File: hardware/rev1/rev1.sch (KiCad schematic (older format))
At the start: 28 parts, among them U1 BNO055, U2 MPL3115A2, U3 Teensy3.6, Y1 Crystal_32kHz768

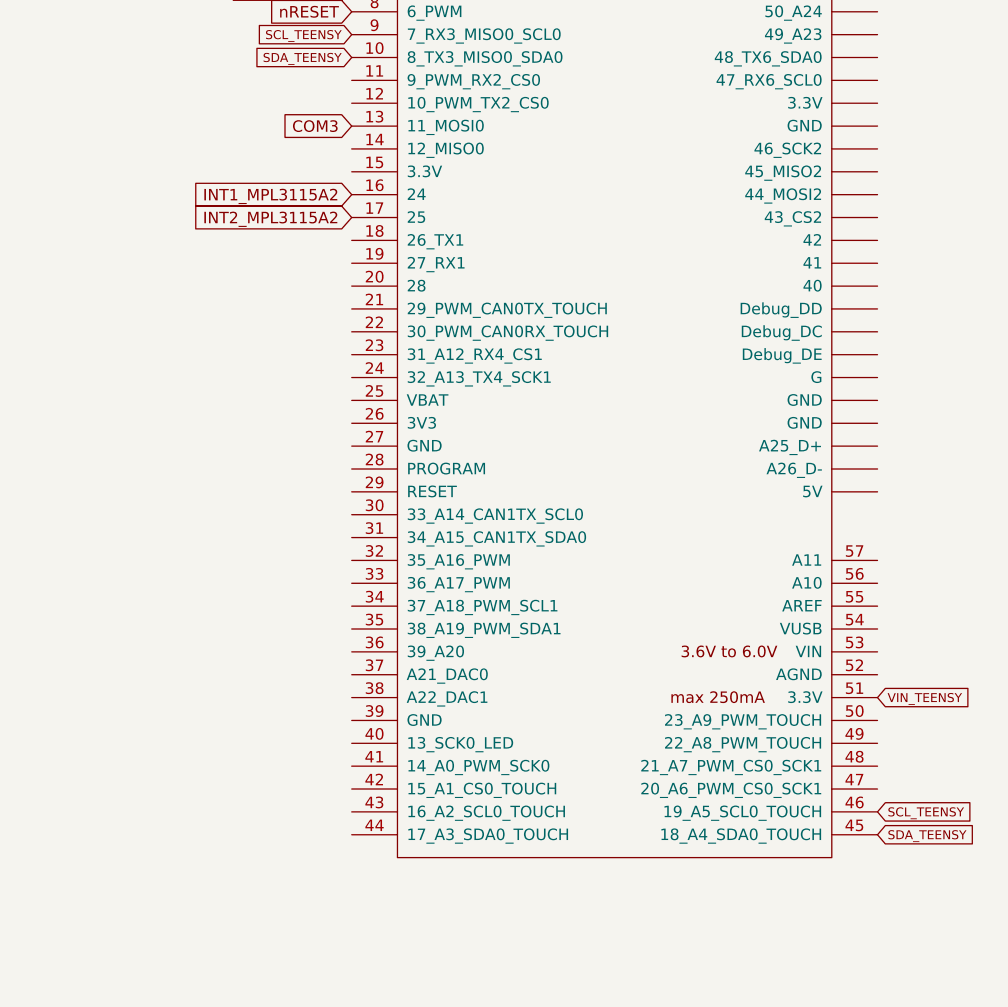
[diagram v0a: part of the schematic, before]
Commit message: wip
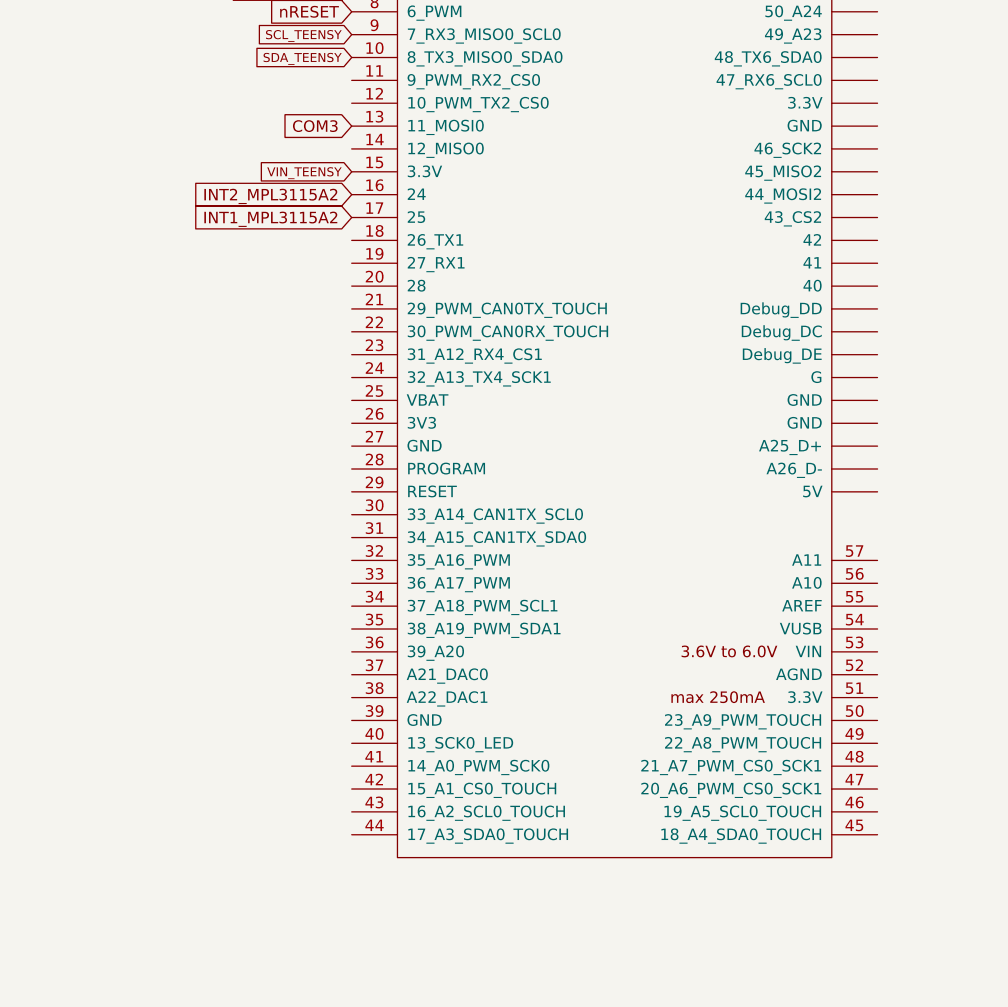
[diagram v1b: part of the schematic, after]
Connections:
- net +3V3: now also U3.15 (3.3V); no longer U3.51 (3.3V)
- net INT1_MPL3115A2: now also U3.17 (25); no longer U3.16 (24)
- net INT2_MPL3115A2: now also U3.16 (24); no longer U3.17 (25)
- net SCL_TEENSY: no longer U3.46 (19_A5_SCL0_TOUCH)
- net SDA_TEENSY: no longer U3.45 (18_A4_SDA0_TOUCH)
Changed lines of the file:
@@
 Text Label 27400 2800 2    118  ~ 0
 GND
-Text GLabel 29700 6500 2    39   Input ~ 0
+Text GLabel 27400 4200 0    39   Input ~ 0
 VIN_TEENSY
-Text GLabel 29700 7100 2    39   Input ~ 0
-SDA_TEENSY
-Text GLabel 29700 7000 2    39   Input ~ 0
-SCL_TEENSY
 Wire Wire Line
 	6900 7300 9850 7300
 Text GLabel 9850 7300 2    50   Input ~ 0
 INT_BNO055
+Text GLabel 27400 4400 0    50   Input ~ 0
+INT1_MPL3115A2
 Text GLabel 27400 4300 0    50   Input ~ 0
-INT1_MPL3115A2
-Text GLabel 27400 4400 0    50   Input ~ 0
 INT2_MPL3115A2
 Text GLabel 27400 3500 0    50   Input ~ 0
